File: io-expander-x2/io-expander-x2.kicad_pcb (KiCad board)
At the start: 2 copper layers, 50 x 100 mm, 6 parts, among them IC1 MCP23017-E_SO, IC2 MCP23017-E_SO, J1 CONN4_BM04B-SRSS_JST, J2 CONN4_BM04B-SRSS_JST, J3 Screw-8P-5.08-1729186, J4 Screw-8P-5.08-1729186

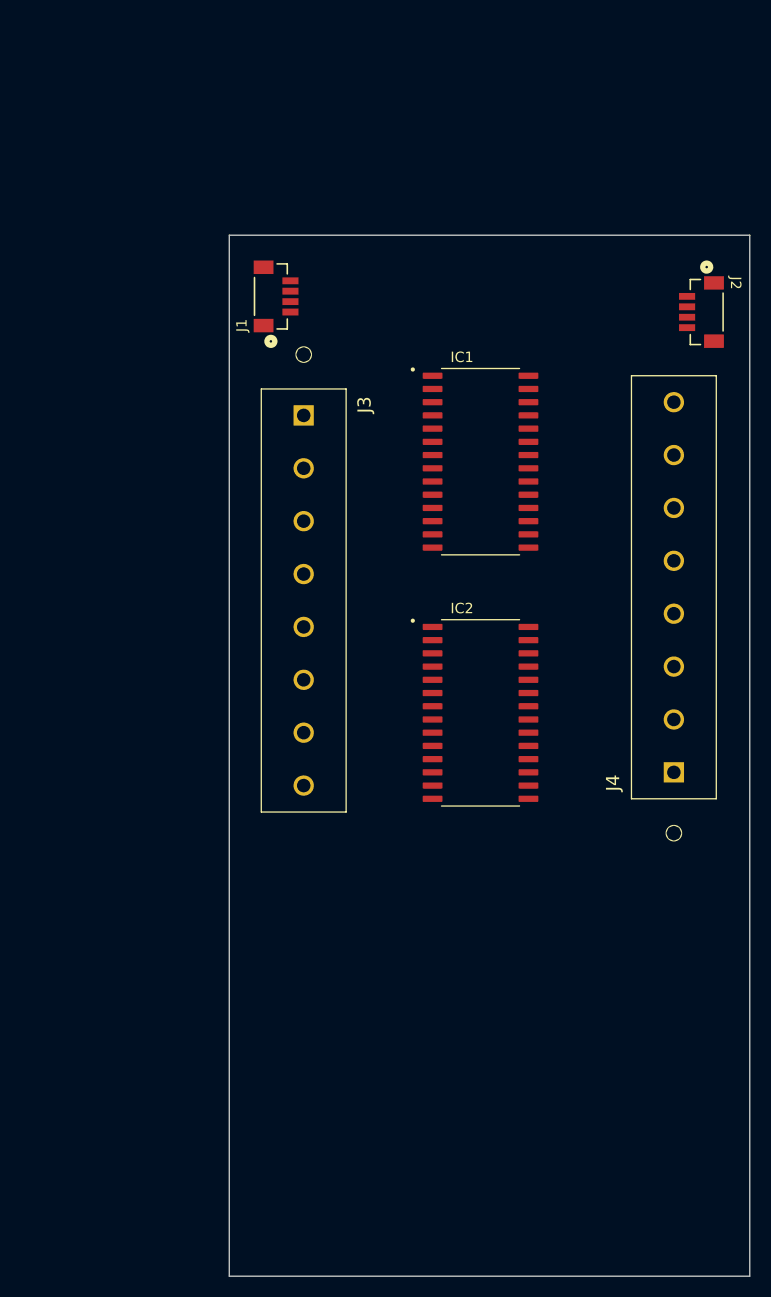
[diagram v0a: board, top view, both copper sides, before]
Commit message: Daughter board is coming along nicely.
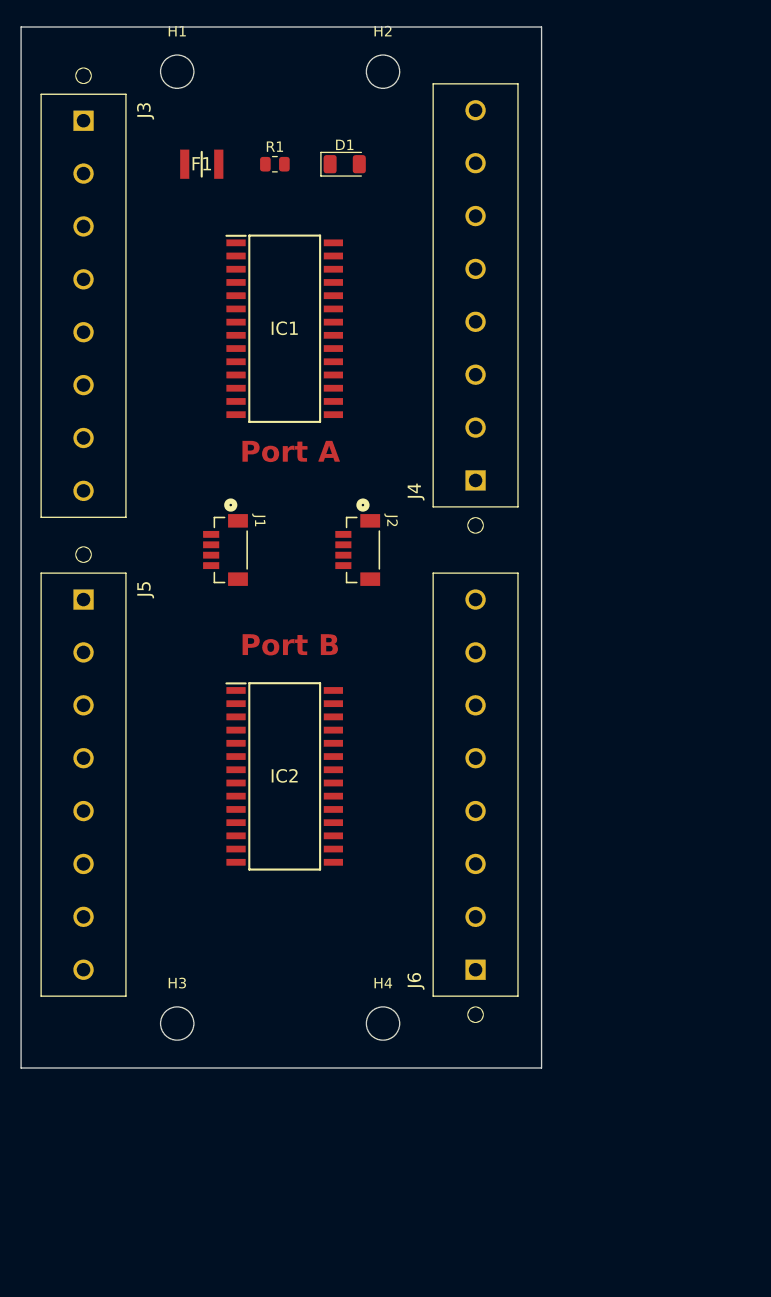
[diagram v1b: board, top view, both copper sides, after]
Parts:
- added D1: LED, LED_SMD:LED_1206_3216Metric, F.Cu at (61.1, 43.2)
- added F1: MF-USHT010KX-2, 00_General:FUSC3226X85N, F.Cu at (47.4, 43.2)
- added H1: MountingHole, MountingHole:MountingHole_3.2mm_M3_ISO7380, F.Cu at (45.0, 34.3)
- added H2: MountingHole, MountingHole:MountingHole_3.2mm_M3_ISO7380, F.Cu at (64.8, 34.3)
- added H3: MountingHole, MountingHole:MountingHole_3.2mm_M3_ISO7380, F.Cu at (45.0, 125.7)
- added H4: MountingHole, MountingHole:MountingHole_3.2mm_M3_ISO7380, F.Cu at (64.8, 125.7)
- added J5: Screw-8P-5.08-1729186, 00_Connectors:Screw-8P-5.08-1729186, F.Cu at (36.0, 85.0)
- added J6: Screw-8P-5.08-1729186, 00_Connectors:Screw-8P-5.08-1729186, F.Cu at (73.7, 120.6)
- added R1: R, Resistor_SMD:R_0805_2012Metric, F.Cu at (54.4, 43.2)
- IC1, IC2: footprint 00_General:SOIC127P1030X265-28N -> SamacSys_Parts:SOIC127P1030X265-28N
- moved J2 40.2 mm to (62.8, 80.2)
- moved J3 35.3 mm to (36.0, 39.0)
- moved J4 33.9 mm to (73.7, 73.6)
- moved J1 24.7 mm to (50.1, 80.2), turned to -90 degrees
- moved IC1 22.7 mm to (55.3, 59.0)
- moved IC2 19.8 mm to (55.3, 102.0)
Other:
- board text added: "Port A"
- board text added: "Port B"
